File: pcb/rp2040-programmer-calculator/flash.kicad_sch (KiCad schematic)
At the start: 5 parts, among them SW64 PTS636SL50 LFS, U7 W25Q32JVSS

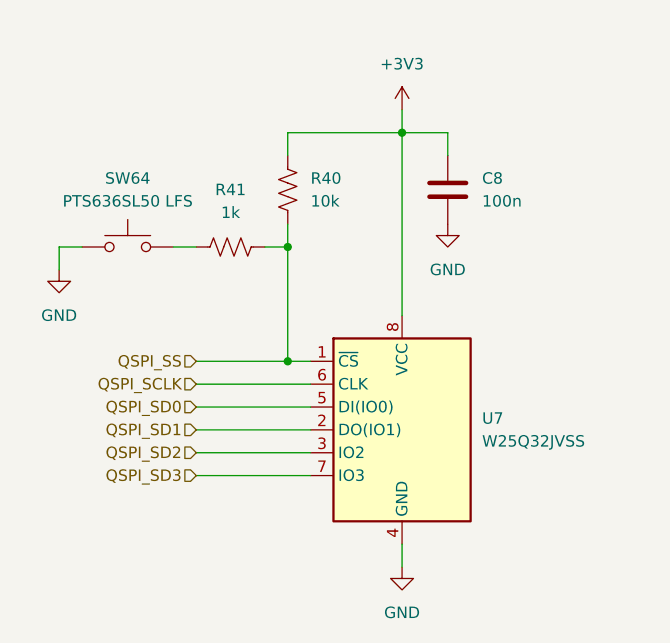
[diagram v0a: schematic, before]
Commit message: Finished design
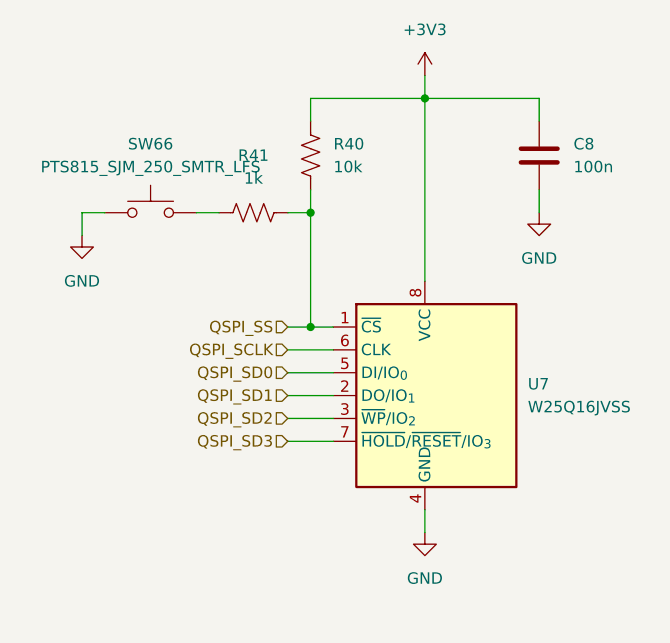
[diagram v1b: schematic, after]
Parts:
- removed SW64: PTS636SL50 LFS, SamacSys_Parts:PTS636SL50LFS, symbol Switch:SW_Push
- removed U7: W25Q32JVSS, Package_SO:SOIC-8_5.23x5.23mm_P1.27mm, symbol Memory_Flash:W25Q32JVSS
- added SW66: PTS815_SJM_250_SMTR_LFS, PTS815_SJM_250_SMTR_LFS:SW_Push_PTS815_SJM_250_SMTR_LFS, symbol Switch:SW_Push
- added U7: W25Q16JVSS, Package_SO:SOIC-8_5.3x5.3mm_P1.27mm, symbol Memory_Flash:W25Q16JVSS
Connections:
- net +3V3: now also U7.8 (VCC)
- net GND: now also SW66.1, U7.4 (GND)
- net QSPI_SCLK: now also U7.6 (CLK)
- net QSPI_SD0: now also U7.5 (DI/IO_{0})
- net QSPI_SD1: now also U7.2 (DO/IO_{1})
- net QSPI_SD2: now also U7.3 (~{WP}/IO_{2})
- net QSPI_SD3: now also U7.7 (~{HOLD}/~{RESET}/IO_{3})
- net QSPI_SS: now also U7.1 (~{CS})
- net at R41.1: now also SW66.2
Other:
- moved on the sheet: C8, R40, R41
